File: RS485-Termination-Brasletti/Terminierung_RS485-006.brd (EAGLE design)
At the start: 14 x 23 mm, 9 parts, among them IC1 REG1117, X1 1751264

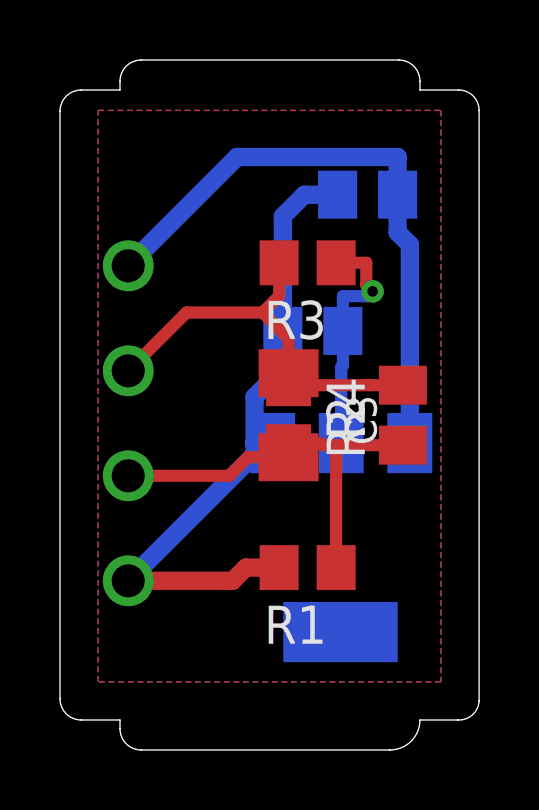
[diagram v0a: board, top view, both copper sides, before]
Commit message: Rs485 Term
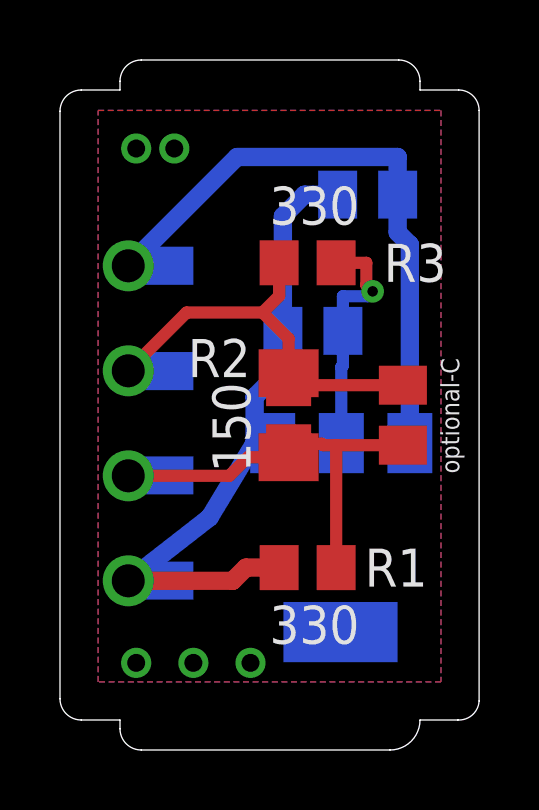
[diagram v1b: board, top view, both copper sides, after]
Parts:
- added PAD1, PAD2, PAD3, PAD4: WIREPADSMD1,27-254, wirepad:SMD1,27-2,54
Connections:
- removed net N$3: C3.1, R1.1, R2.2, R4.2, X1.3
- removed net N$4: C3.2, R2.1, R3.2, R4.1, X1.2
- new net A: C3.2, PAD2.1, R2.1, R3.2, R4.1, X1.2
- new net B: C3.1, PAD3.1, R1.1, R2.2, R4.2, X1.3
- net GND: now also PAD4.1
- net VCC: now also PAD1.1
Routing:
- net N$3: track 14.1 -> 0.00 mm
- net B: track 0.00 -> 14.1 mm
- net N$4: track 13.8 -> 0.00 mm
- net A: track 0.00 -> 13.8 mm
- net GND: vias 0 -> 5
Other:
- board text added: "100uF"
- board text added: "10uF"
- board text added: "150"
- board text added: "330"
- board text added: "A"
- board text added: "AMS1117"
- board text added: "B"
- board text added: "C1"
- board text added: "C2"
- board text added: "GND"
- board text added: "R1"
- board text added: "R2"
- board text added: "R3"
- board text added: "VCC"
- board text added: "optional-C"
